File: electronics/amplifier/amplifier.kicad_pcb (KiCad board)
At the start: 2 copper layers, 170.9 x 93.2 mm, 96 parts, among them K1 FRT5_separated, K2 FRT5_separated, K4 screw_terminal_2x01, P1 CONN_02X01, P2 CONN_02X01, P3 CONN_02X01, P4 CONN_02X01, P5 CONN_01X03, Q1 BC548, Q4 BC548, Q5 BC548, U1 LM1875, U2 TL082, U3 LM7815CT, U4 CK6418, U5 LM7805CT, U6 CK6418, U7 LM1875

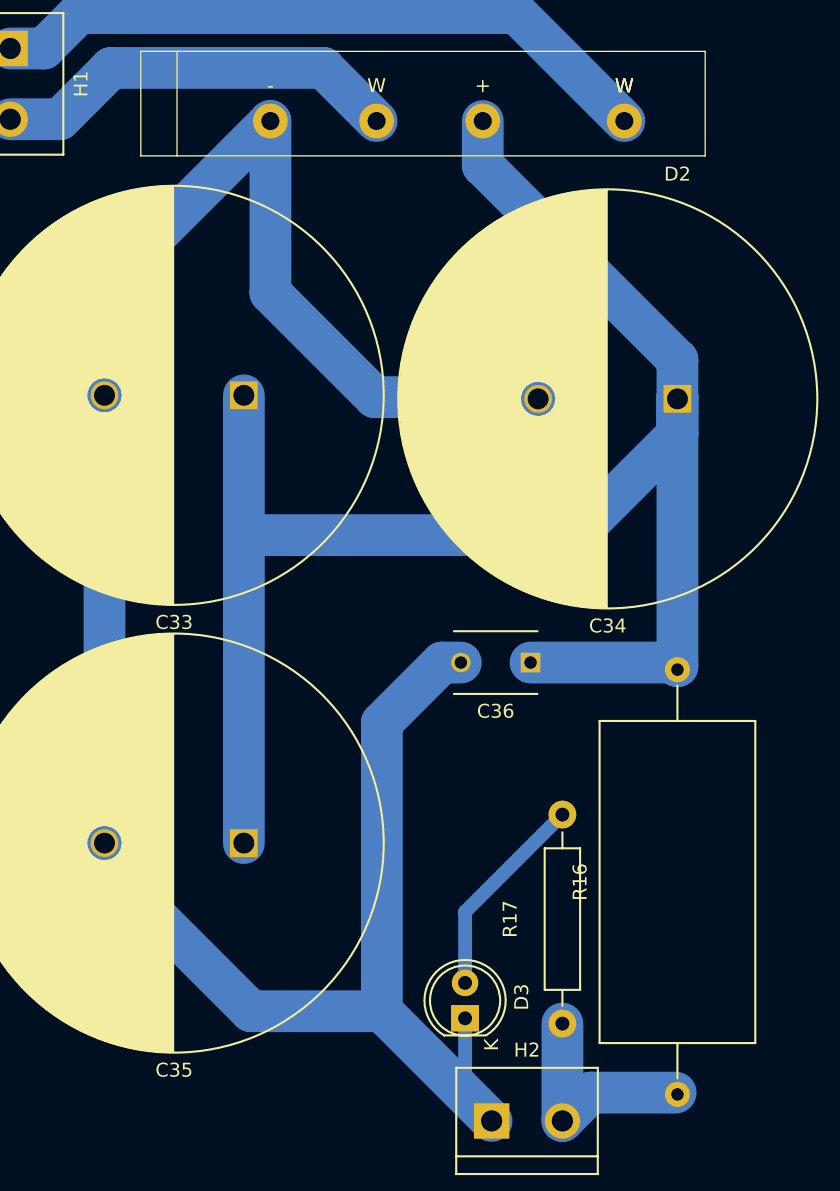
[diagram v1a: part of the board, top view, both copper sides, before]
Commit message: changed some parts
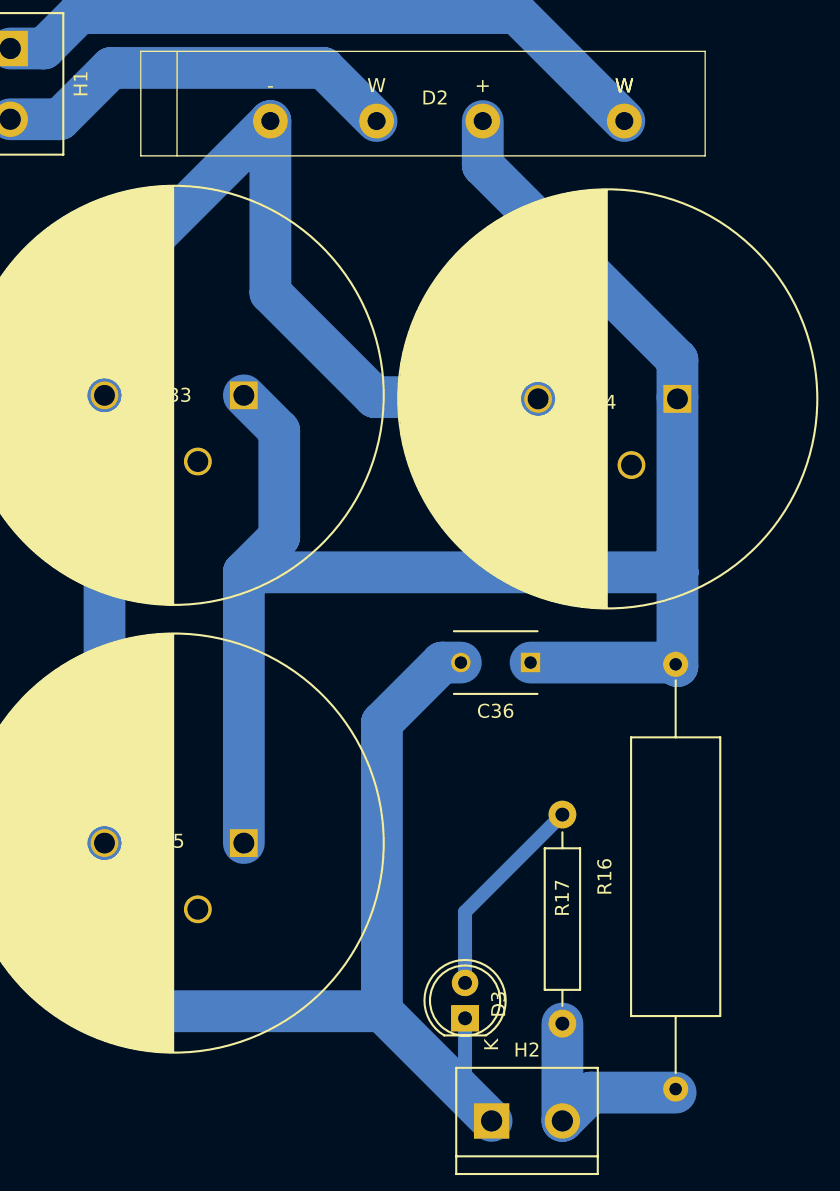
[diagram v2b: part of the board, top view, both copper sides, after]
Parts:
- C33, C34, C35: footprint Capacitors_ThroughHole:C_Radial_D30_L51_P10 -> special_symbols:C_Radial_D30_L51_P10_3pin
- D2: value Diode_Bridge -> B40C5000
- R16: footprint Resistors_ThroughHole:Resistor_Ceramic_Horizontal_L23mm-W9mm-H9mm-p30mm -> special_symbols:Resistor_Ceramic_Horizontal_L25mm-W6.4mm-H6.4mm-p30mm
- moved R16 0.40 mm to (89.9, 101.6)
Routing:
- net Net-(C33-Pad2): track 164.6 -> 168.8 mm
- net Net-(C33-Pad1): track 124.5 -> 121.2 mm
